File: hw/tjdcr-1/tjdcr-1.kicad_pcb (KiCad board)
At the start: 2 copper layers, 100.2 x 35 mm, 32 parts, among them J1 Conn_Coaxial, J2 Tuning Inductor, J3 Power, J4 LO Option, Q1 MMBT3904, Q2 MMBFJ310, T1 5:28, T2 28:5, T3 Transformer_1P_2S, T4 Transformer_1P_2S

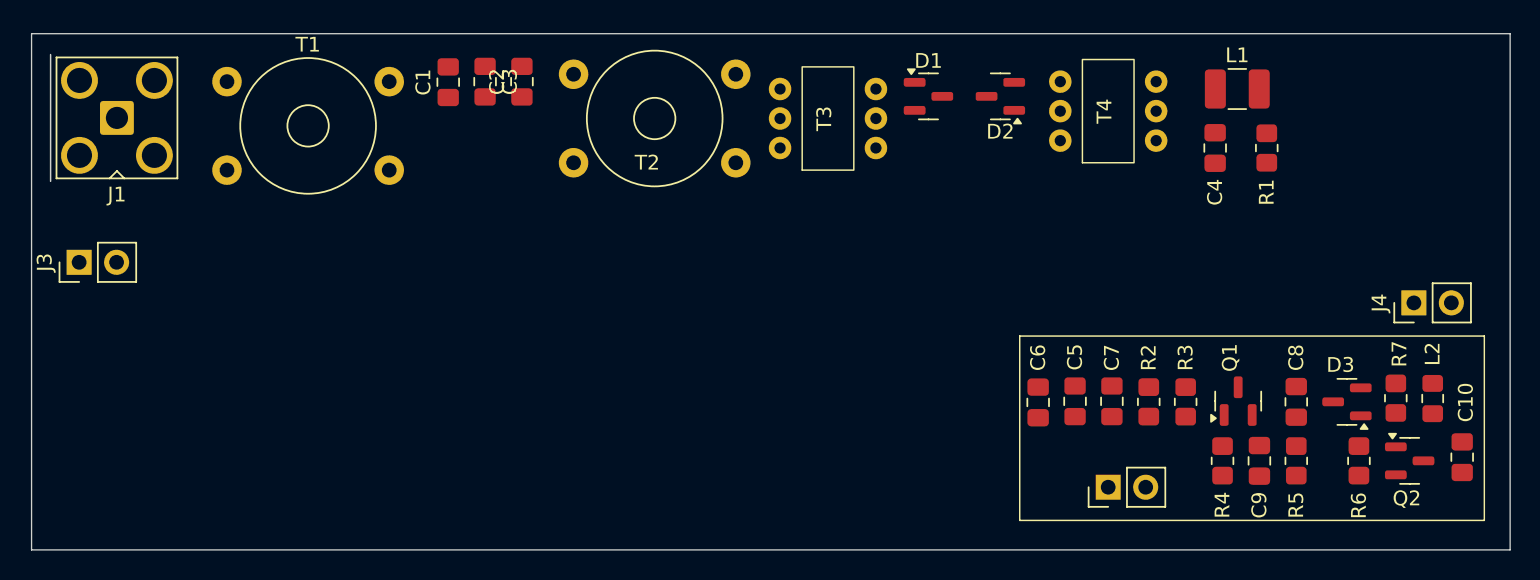
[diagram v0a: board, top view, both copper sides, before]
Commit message: Layout is progressing
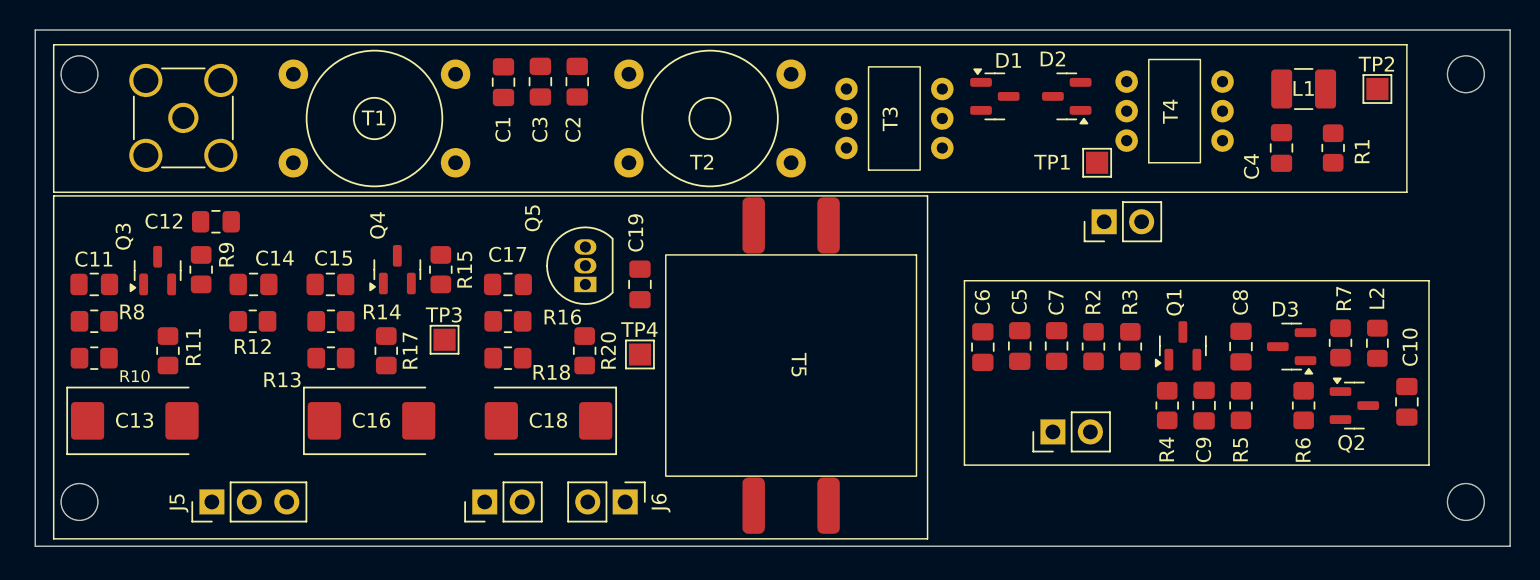
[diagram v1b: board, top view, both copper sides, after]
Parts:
- added C11: 0.1u, Capacitor_SMD:C_0805_2012Metric_Pad1.18x1.45mm_HandSolder, F.Cu at (78.0, 68.2)
- added C12: 47u, Capacitor_SMD:C_0805_2012Metric_Pad1.18x1.45mm_HandSolder, F.Cu at (86.2, 64.0)
- added C13: 470u (Size 2917/7343), Capacitor_Tantalum_SMD:CP_EIA-7343-20_Kemet-V_Pad2.25x2.55mm_HandSolder, F.Cu at (80.8, 77.5)
- added C14: 47u, Capacitor_SMD:C_0805_2012Metric_Pad1.18x1.45mm_HandSolder, F.Cu at (88.8, 68.2)
- added C15: 10u, Capacitor_SMD:C_0805_2012Metric_Pad1.18x1.45mm_HandSolder, F.Cu at (94.0, 68.2)
- added C16: 470u (Size 2917/7343), Capacitor_Tantalum_SMD:CP_EIA-7343-20_Kemet-V_Pad2.25x2.55mm_HandSolder, F.Cu at (96.8, 77.5)
- added C17: 10u, Capacitor_SMD:C_0805_2012Metric_Pad1.18x1.45mm_HandSolder, F.Cu at (106.0, 68.2)
- added C18: 470u (Size 2917/7343), Capacitor_Tantalum_SMD:CP_EIA-7343-20_Kemet-V_Pad2.25x2.55mm_HandSolder, F.Cu at (108.8, 77.5)
- added C19: 47u, Capacitor_SMD:C_0805_2012Metric_Pad1.18x1.45mm_HandSolder, F.Cu at (115.0, 68.2)
- added H1: MountingHole, MountingHole:MountingHole_2.5mm, F.Cu at (77.0, 54.0)
- added H2: MountingHole, MountingHole:MountingHole_2.5mm, F.Cu at (77.0, 83.0)
- added H3: MountingHole, MountingHole:MountingHole_2.5mm, F.Cu at (171.0, 54.0)
- added H4: MountingHole, MountingHole:MountingHole_2.5mm, F.Cu at (171.0, 83.0)
- added J5: Volume, Connector_PinHeader_2.54mm:PinHeader_1x03_P2.54mm_Vertical, F.Cu at (86.0, 83.0)
- added J6: Speaker, Connector_PinHeader_2.54mm:PinHeader_1x02_P2.54mm_Vertical, F.Cu at (114.0, 83.0)
- added Q3: MMBT3904, Package_TO_SOT_SMD:SOT-23, F.Cu at (82.3, 67.3)
- added Q4: MMBT3904, Package_TO_SOT_SMD:SOT-23, F.Cu at (98.5, 67.2)
- added Q5: 2N3904, Package_TO_SOT_THT:TO-92_Inline, F.Cu at (111.3, 68.2)
- added R10: 4.7k, Resistor_SMD:R_0805_2012Metric_Pad1.20x1.40mm_HandSolder, F.Cu at (78.0, 73.2)
- added R11: 470, Resistor_SMD:R_0805_2012Metric_Pad1.20x1.40mm_HandSolder, F.Cu at (83.0, 72.8)
- added R12: 220, Resistor_SMD:R_0805_2012Metric_Pad1.20x1.40mm_HandSolder, F.Cu at (88.8, 70.8)
- added R13: 4.7k, Resistor_SMD:R_0805_2012Metric_Pad1.20x1.40mm_HandSolder, F.Cu at (94.0, 73.2)
- added R14: 14.7k, Resistor_SMD:R_0805_2012Metric_Pad1.20x1.40mm_HandSolder, F.Cu at (94.0, 70.8)
- added R15: 1k, Resistor_SMD:R_0805_2012Metric_Pad1.20x1.40mm_HandSolder, F.Cu at (101.5, 67.2)
- added R16: 14.7k, Resistor_SMD:R_0805_2012Metric_Pad1.20x1.40mm_HandSolder, F.Cu at (106.0, 70.8)
- added R17: 470, Resistor_SMD:R_0805_2012Metric_Pad1.20x1.40mm_HandSolder, F.Cu at (97.8, 72.8)
- added R18: 4.7k, Resistor_SMD:R_0805_2012Metric_Pad1.20x1.40mm_HandSolder, F.Cu at (106.0, 73.2)
- added R20: 10, Resistor_SMD:R_0805_2012Metric_Pad1.20x1.40mm_HandSolder, F.Cu at (111.2, 72.8)
- added R8: 14.7k, Resistor_SMD:R_0805_2012Metric_Pad1.20x1.40mm_HandSolder, F.Cu at (78.0, 70.8)
- added R9: 1k, Resistor_SMD:R_0805_2012Metric_Pad1.20x1.40mm_HandSolder, F.Cu at (85.2, 67.2)
- added T5: Transformer_1P_1S, bruce-footprints:CheapAudioTransformer, F.Cu at (125.2, 73.8)
- added TP1: TestPoint, TestPoint:TestPoint_Pad_1.5x1.5mm, F.Cu at (146.0, 60.0)
- added TP2: TestPoint, TestPoint:TestPoint_Pad_1.5x1.5mm, F.Cu at (165.0, 55.0)
- added TP3: TestPoint, TestPoint:TestPoint_Pad_1.5x1.5mm, F.Cu at (101.8, 72.0)
- added TP4: TestPoint, TestPoint:TestPoint_Pad_1.5x1.5mm, F.Cu at (115.0, 73.0)
- J1: footprint Connector_Coaxial:SMA_Amphenol_901-143_Horizontal -> Connector_Coaxial:SMA_Amphenol_901-144_Vertical
- J2: value Tuning Inductor -> Tuning
- moved J3 31.9 mm to (104.5, 83.0)
- moved J4 21.7 mm to (146.5, 64.0)
- moved C10 5.30 mm to (167.0, 76.2)
- moved C5 5.30 mm to (140.8, 72.4)
- moved C6 5.30 mm to (138.2, 72.5)
- moved C7 5.30 mm to (143.2, 72.4)
- moved C8 5.30 mm to (155.8, 72.5)
- moved C9 5.30 mm to (153.2, 76.5)
- moved D3 5.30 mm to (159.2, 72.5)
- moved J2 5.30 mm to (143.0, 78.2)
- moved L2 5.30 mm to (165.0, 72.2)
- moved Q1 5.30 mm to (151.8, 72.4)
- moved Q2 5.30 mm to (163.4, 76.5)
- moved R2 5.30 mm to (145.8, 72.5)
- moved R3 5.30 mm to (148.2, 72.5)
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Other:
- board size 100.2 x 35 mm -> 100 x 35 mm
